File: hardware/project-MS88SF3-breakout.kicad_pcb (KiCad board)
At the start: 4 copper layers, 22.9 x 50.8 mm, 28 parts, among them J1 Conn_02x05_Odd_Even, J2 S2B-PH-SM4-TB(LF)(SN), J3 USB4105-GF-A, J4 Conn_01x12_Male, J5 Conn_01x16_Male, U1 MS88SF3_NRF52840

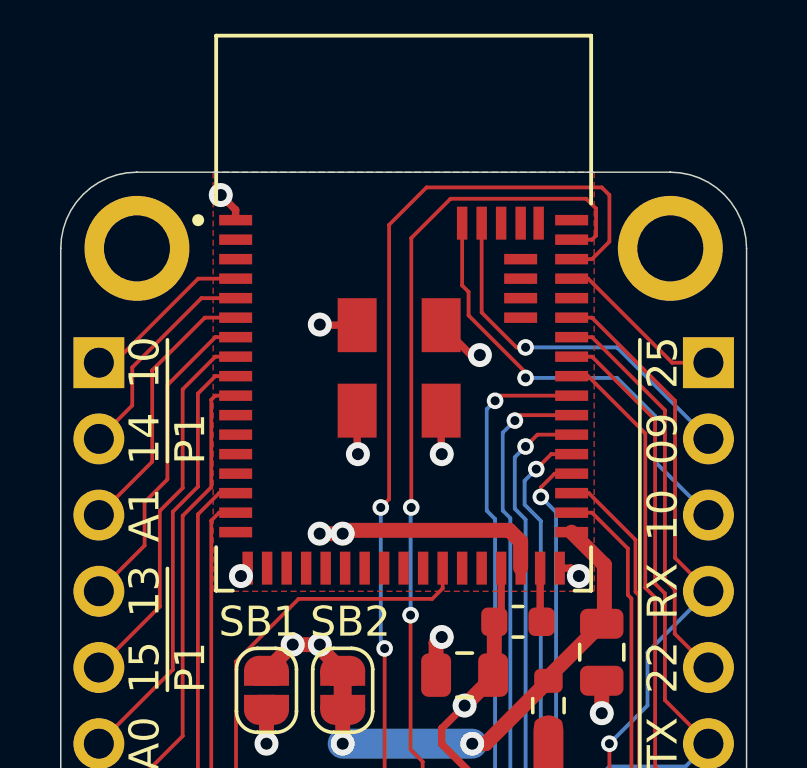
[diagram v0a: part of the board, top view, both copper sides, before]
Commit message: Upgrade ground fill under module
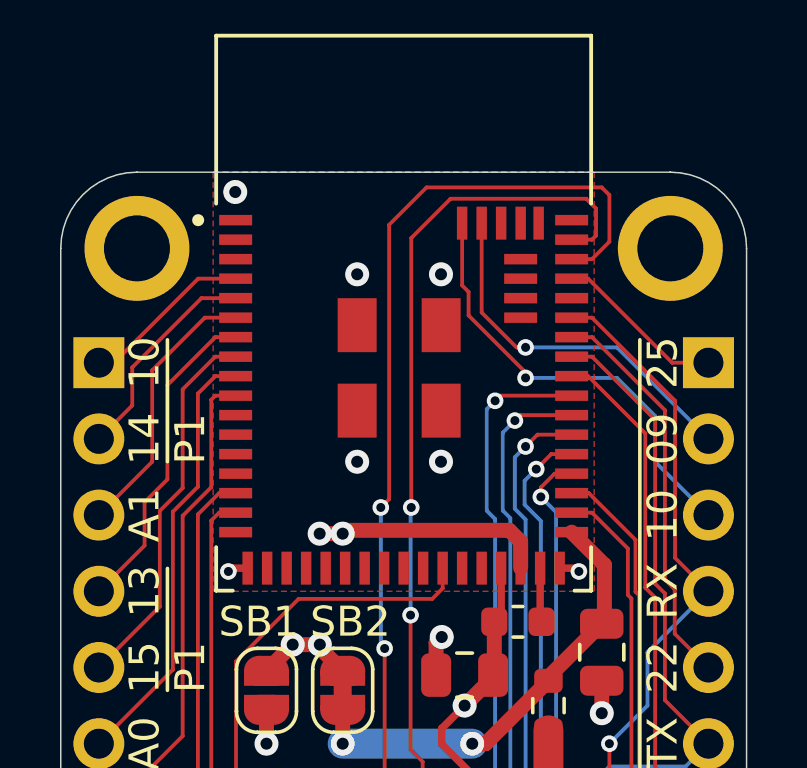
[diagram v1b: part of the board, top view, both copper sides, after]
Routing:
- net GND: track 36.1 -> 29.5 mm
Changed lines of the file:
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@@
     (thickness 1.6)
     (drawings 53)
-    (tracks 396)
+    (tracks 386)
     (zones 0)
     (modules 28)
@@
     )
   )
-  (module MS88SF3_NRF52840:MODULE_MS88SF3_NRF52840 (layer F.Cu)
+  (module MS88SF3_NRF52840:MODULE_MS88SF3_NRF52840 locked (layer F.Cu)
     (at 47.498 85.471)
     (fp_text reference U1 (at -3.325 10.635) (layer F.Fab) hide
@@
     )
   )
-  (module Connector_PinHeader_2.54mm:PinHeader_1x12_P2.54mm_Vertical (layer B.Cu)
+  (module Connector_PinHeader_2.54mm:PinHeader_1x12_P2.54mm_Vertical locked (layer B.Cu)
     (at 37.338 87.122 180)
     (descr "Through hole straight pin header, 1x12, 2.54mm pitch, single row")
@@
     )
   )
-  (module USB4105-GF-A:GCT_USB4105-GF-A (layer F.Cu)
+  (module USB4105-GF-A:GCT_USB4105-GF-A locked (layer F.Cu)
     (at 47.498 130.302)
     (fp_text reference J3 (at -1.27 -6.858) (layer F.Fab) hide
@@
     )
   )
-  (module Connector_PinHeader_2.54mm:PinHeader_1x16_P2.54mm_Vertical (layer B.Cu)
+  (module Connector_PinHeader_2.54mm:PinHeader_1x16_P2.54mm_Vertical locked (layer B.Cu)
     (at 57.658 87.122 180)
     (descr "Through hole straight pin header, 1x16, 2.54mm pitch, single row")
@@
       (net 20 /RESET))
   )
-  (module "S2B-PH-SM4-TB(LF)(SN):JST_S2B-PH-SM4-TB(LF)(SN)" (layer F.Cu)
+  (module "S2B-PH-SM4-TB(LF)(SN):JST_S2B-PH-SM4-TB(LF)(SN)" locked (layer F.Cu)
     (at 43.688 120.777 270)
     (fp_text reference J2 (at -0.69228 -3.184 90) (layer F.Fab) hide
@@
     )
   )
-  (module MountingHole:MountingHole_2.2mm_M2_ISO7380_Pad (layer F.Cu)
+  (module MountingHole:MountingHole_2.2mm_M2_ISO7380_Pad locked (layer F.Cu)
     (at 56.388 83.312)
     (descr "Mounting Hole 2.2mm, M2, ISO7380")
@@
       (net 7 GND))
   )
-  (module MountingHole:MountingHole_2.2mm_M2_ISO7380_Pad (layer F.Cu)
+  (module MountingHole:MountingHole_2.2mm_M2_ISO7380_Pad locked (layer F.Cu)
     (at 38.608 83.312)
     (descr "Mounting Hole 2.2mm, M2, ISO7380")
@@
   (via (at 51.308 116.332) (size 0.8) (drill 0.4) (layers F.Cu B.Cu) (net 7))
   (segment (start 51.308 117.285) (end 51.308 116.332) (width 0.25) (layer F.Cu) (net 7))
-  (via (at 45.974 90.17) (size 0.8) (drill 0.4) (layers F.Cu B.Cu) (net 7))
-  (segment (start 45.948 88.721) (end 45.948 90.144) (width 0.25) (layer F.Cu) (net 7))
-  (segment (start 45.948 90.144) (end 45.974 90.17) (width 0.25) (layer F.Cu) (net 7))
-  (segment (start 52.698 93.971) (end 53.077 93.971) (width 0.25) (layer F.Cu) (net 7))
-  (via (at 53.34 94.234) (size 0.8) (drill 0.4) (layers F.Cu B.Cu) (net 7))
-  (segment (start 53.077 93.971) (end 53.34 94.234) (width 0.25) (layer F.Cu) (net 7))
   (segment (start 52.7215 127.0255) (end 51.818 126.122) (width 0.25) (layer F.Cu) (net 7))
   (segment (start 53.848 127.0255) (end 52.7215 127.0255) (width 0.25) (layer F.Cu) (net 7))
-  (via (at 42.075019 94.234) (size 0.8) (drill 0.4) (layers F.Cu B.Cu) (net 7))
-  (segment (start 42.298 93.971) (end 42.075019 94.193981) (width 0.25) (layer F.Cu) (net 7))
-  (segment (start 42.075019 94.193981) (end 42.075019 94.234) (width 0.25) (layer F.Cu) (net 7))
   (via (at 44.958 103.886) (size 0.8) (drill 0.4) (layers F.Cu B.Cu) (net 7))
   (segment (start 44.958 101.936) (end 44.958 103.886) (width 0.5) (layer F.Cu) (net 7))
@@
   (via (at 46.482 112.776) (size 0.554) (drill 0.3) (layers F.Cu B.Cu) (net 7))
   (segment (start 46.482 111.773) (end 46.482 112.776) (width 0.25) (layer F.Cu) (net 7))
-  (segment (start 48.748 88.721) (end 48.748 90.15) (width 0.25) (layer F.Cu) (net 7))
-  (via (at 48.768 90.17) (size 0.8) (drill 0.4) (layers F.Cu B.Cu) (net 7))
-  (segment (start 48.748 90.15) (end 48.768 90.17) (width 0.25) (layer F.Cu) (net 7))
-  (segment (start 44.723 85.871) (end 44.704 85.852) (width 0.25) (layer F.Cu) (net 7))
-  (segment (start 45.948 85.871) (end 44.723 85.871) (width 0.25) (layer F.Cu) (net 7))
-  (via (at 44.704 85.852) (size 0.8) (drill 0.4) (layers F.Cu B.Cu) (net 7))
-  (via (at 50.037976 86.868) (size 0.8) (drill 0.4) (layers F.Cu B.Cu) (net 7))
-  (segment (start 48.748 85.871) (end 49.745 86.868) (width 0.25) (layer F.Cu) (net 7))
-  (segment (start 49.745 86.868) (end 50.037976 86.868) (width 0.25) (layer F.Cu) (net 7))
-  (via (at 41.402014 81.534) (size 0.8) (drill 0.4) (layers F.Cu B.Cu) (net 7))
-  (segment (start 41.898 82.029986) (end 41.402014 81.534) (width 0.25) (layer F.Cu) (net 7))
-  (segment (start 41.898 82.371) (end 41.898 82.029986) (width 0.25) (layer F.Cu) (net 7))
+  (via (at 41.8846 81.4324) (size 0.8) (drill 0.4) (layers F.Cu B.Cu) (net 7))
+  (via (at 53.34 94.0816) (size 0.554) (drill 0.3) (layers F.Cu B.Cu) (net 7))
+  (segment (start 52.698 93.971) (end 53.2294 93.971) (width 0.25) (layer F.Cu) (net 7))
+  (segment (start 53.2294 93.971) (end 53.34 94.0816) (width 0.25) (layer F.Cu) (net 7))
+  (via (at 41.656 94.0816) (size 0.554) (drill 0.3) (layers F.Cu B.Cu) (net 7))
+  (segment (start 41.7666 93.971) (end 42.298 93.971) (width 0.25) (layer F.Cu) (net 7))
+  (segment (start 41.656 94.0816) (end 41.7666 93.971) (width 0.25) (layer F.Cu) (net 7))
+  (via (at 48.7426 84.1756) (size 0.8) (drill 0.4) (layers F.Cu B.Cu) (net 7))
+  (via (at 45.9486 84.1756) (size 0.8) (drill 0.4) (layers F.Cu B.Cu) (net 7))
+  (via (at 45.9486 90.424) (size 0.8) (drill 0.4) (layers F.Cu B.Cu) (net 7))
+  (via (at 48.7426 90.424) (size 0.8) (drill 0.4) (layers F.Cu B.Cu) (net 7))
   (segment (start 56.544499 88.390499) (end 56.544499 93.628499) (width 0.127) (layer F.Cu) (net 16))
   (segment (start 56.544499 93.628499) (end 57.658 94.742) (width 0.127) (layer F.Cu) (net 16))
@@
   (segment (start 41.348698 92.121) (end 41.898 92.121) (width 0.127) (layer F.Cu) (net 62))
   (segment (start 41.084499 92.385199) (end 41.348698 92.121) (width 0.127) (layer F.Cu) (net 62))
+  (segment (start 37.338 107.442) (end 41.084499 103.695501) (width 0.127) (layer F.Cu) (net 62))
   (segment (start 41.084499 103.695501) (end 41.084499 92.385199) (width 0.127) (layer F.Cu) (net 62))
-  (segment (start 37.338 107.442) (end 41.084499 103.695501) (width 0.127) (layer F.Cu) (net 62))
   (segment (start 41.348698 91.471) (end 41.898 91.471) (width 0.127) (layer F.Cu) (net 63))
   (segment (start 40.64 92.179698) (end 41.348698 91.471) (width 0.127) (layer F.Cu) (net 63))

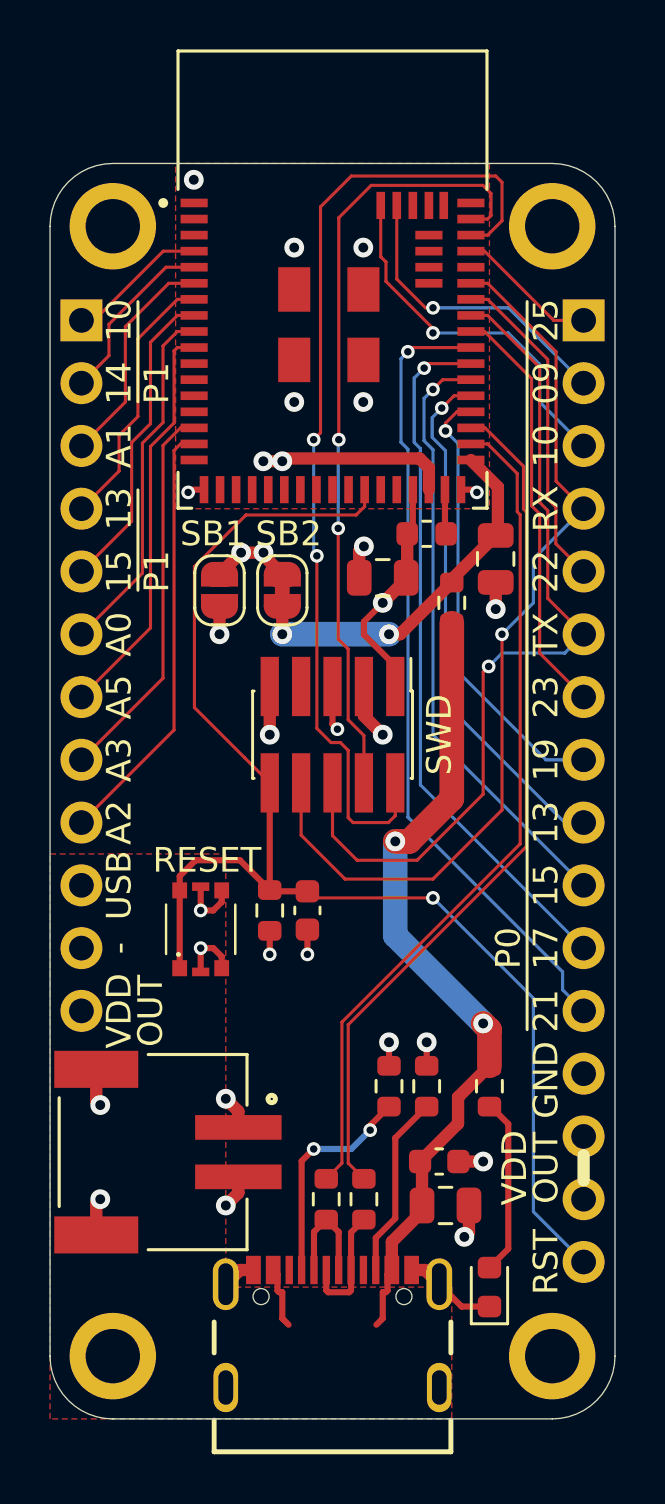
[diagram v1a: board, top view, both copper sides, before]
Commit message: Open pcb and save
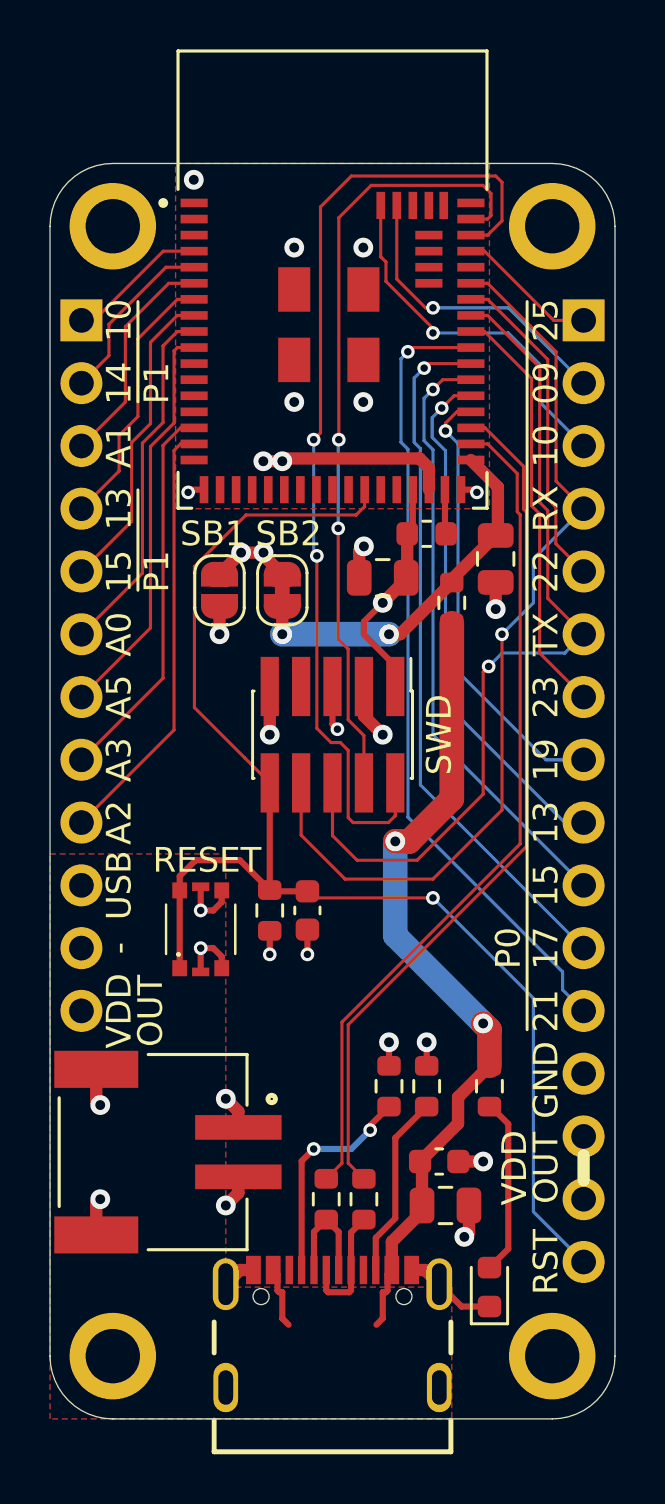
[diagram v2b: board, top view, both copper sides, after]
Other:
- net class Default removed
- net class Smallest removed
